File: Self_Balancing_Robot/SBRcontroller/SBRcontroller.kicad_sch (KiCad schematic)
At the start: 26 parts, among them J1 Conn_01x02, J2 -SW, J3 +SW, J4 +SWLED, J5 -SWLED, U1 THB001P, U11 THB001P, U6 NCP1117-5.0_SOT223, U7 ESP32-DEVKITC

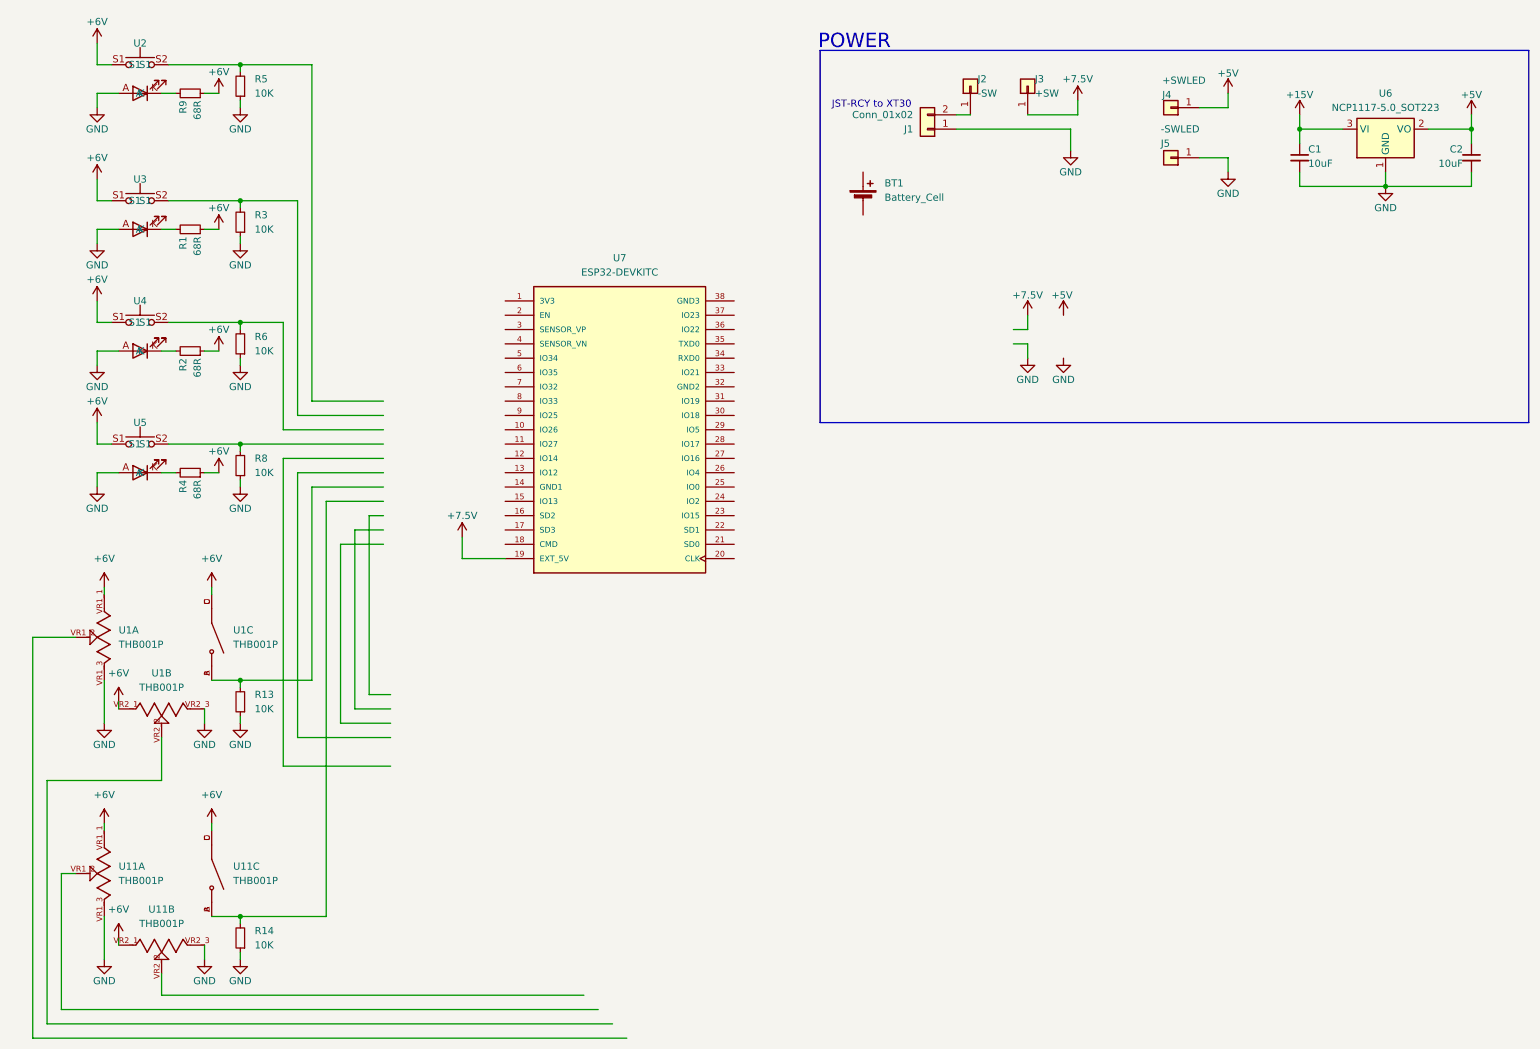
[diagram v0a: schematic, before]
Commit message: sbrcotnrollerm update from windows laptop
dcefefefefe
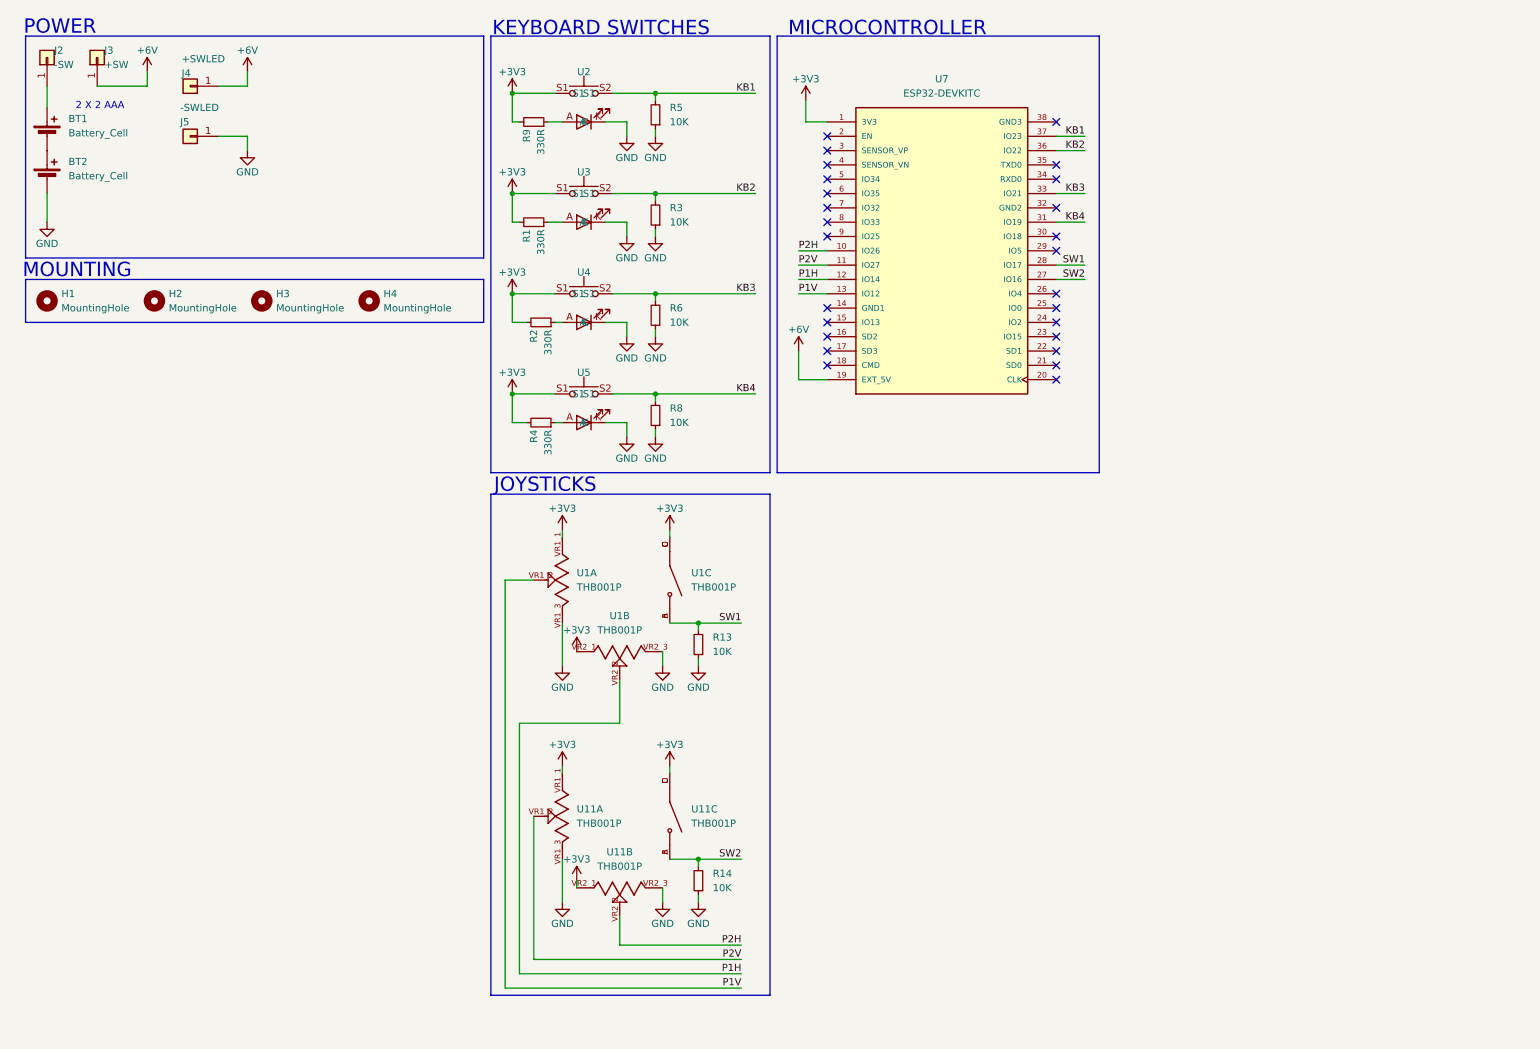
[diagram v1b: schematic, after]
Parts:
- removed C1, C2: 10uF, Capacitor_SMD:C_0805_2012Metric, symbol Device:C_Small
- removed J1: Conn_01x02, Connector_AMASS:AMASS_XT30U-M_1x02_P5.0mm_Vertical, symbol Connector_Generic:Conn_01x02
- removed U6: NCP1117-5.0_SOT223, Package_TO_SOT_SMD:SOT-223-3_TabPin2, symbol Regulator_Linear:NCP1117-5.0_SOT223
- added BT2: Battery_Cell, Battery:BatteryHolder_Keystone_2468_2xAAA, symbol Device:Battery_Cell
- added H1, H2, H3, H4: MountingHole, MountingHole:MountingHole_2.2mm_M2, symbol Mechanical:MountingHole
- BT1: footprint (none) -> Battery:BatteryHolder_Keystone_2468_2xAAA
- J2, J3, J4, J5: footprint SparkFun-Connector:1x01 -> Connector_Wire:SolderWire-1.5sqmm_1x01_D1.7mm_OD3mm
- R1, R2, R4, R9: value 68R -> 330R
- U2, U3, U4, U5: footprint Button_Switch_Keyboard:SW_Cherry_MX_3mmLED -> MX1A-11NN:Cherry_MX_3mmLED
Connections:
- net +5V is gone; now on net +6V: J4.1 (Pin_1)
- net +7.5V is gone; now on net +6V: J3.1 (Pin_1), U7.19 (EXT_5V)
- net +6V: no longer R1.1, R2.1, R4.1, R9.1, U1.C, U1.D, U1.VR1_1, U1.VR2_1, U11.C, U11.D, U11.VR1_1, U11.VR2_1, U2.S1, U3.S1, U4.S1, U5.S1
- net GND: now also U2.K, U3.K, U4.K, U5.K, BT2.2 (-); no longer U2.A, U3.A, U4.A, U5.A
- net +3V3: now reaches R2.2
- net +3V3: now also R1.2, R4.2, R9.2, U1.C, U1.D, U1.VR1_1, U1.VR2_1, U11.C, U11.D, U11.VR1_1, U11.VR2_1, U2.S1, U3.S1, U4.S1, U5.S1, U7.1 (3V3); no longer U4.K
- net KB3: now reaches R6.2, U4.S2 (S1)
- net KB3: now also U7.33 (IO21)
- net KB1: now reaches R5.2, U2.S2 (S1)
- net KB1: now also U7.37 (IO23)
- net SW2: now reaches R14.2, U11.A, U11.B
- net SW2: now also U7.27 (IO16)
- net SW1: now reaches R13.2, U1.A, U1.B
- net SW1: now also U7.28 (IO17)
- net KB4: now reaches R8.2, U5.S2 (S1)
- net KB4: now also U7.31 (IO19)
- net P2V: now reaches U11.VR1_2
- net P2V: now also U7.11 (IO27)
- net P2H: now reaches U7.10 (IO26)
- net P2H: now also U11.VR2_2
- net P1H: now reaches U7.12 (IO14)
- net P1H: now also U1.VR2_2
- net P1V: now reaches U7.13 (IO12)
- net P1V: now also U1.VR1_2
- net KB2: now reaches U7.36 (IO22)
- net KB2: now also R3.2, U3.S2 (S1)
- net at J2.1 (Pin_1): now also BT1.1 (+)
- net at BT1.2 (-): now also BT2.1 (+)
- new net: R2.1, U4.A
- new net: R1.1, U3.A
- new net: R4.1, U5.A
- new net: R9.1, U2.A
- no-connect marks 0 -> 26
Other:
- note added: "2 X 2 AAA"
- note added: "JOYSTICKS"
- note added: "KEYBOARD SWITCHES"
- note added: "MICROCONTROLLER"
- note added: "MOUNTING"
- note removed: "JST-RCY to XT30"
- moved on the sheet: J2, J3, J4, J5, R1, R13, R14, R2, R3, R4, R5, R6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
